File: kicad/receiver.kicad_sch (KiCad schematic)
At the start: 0 parts

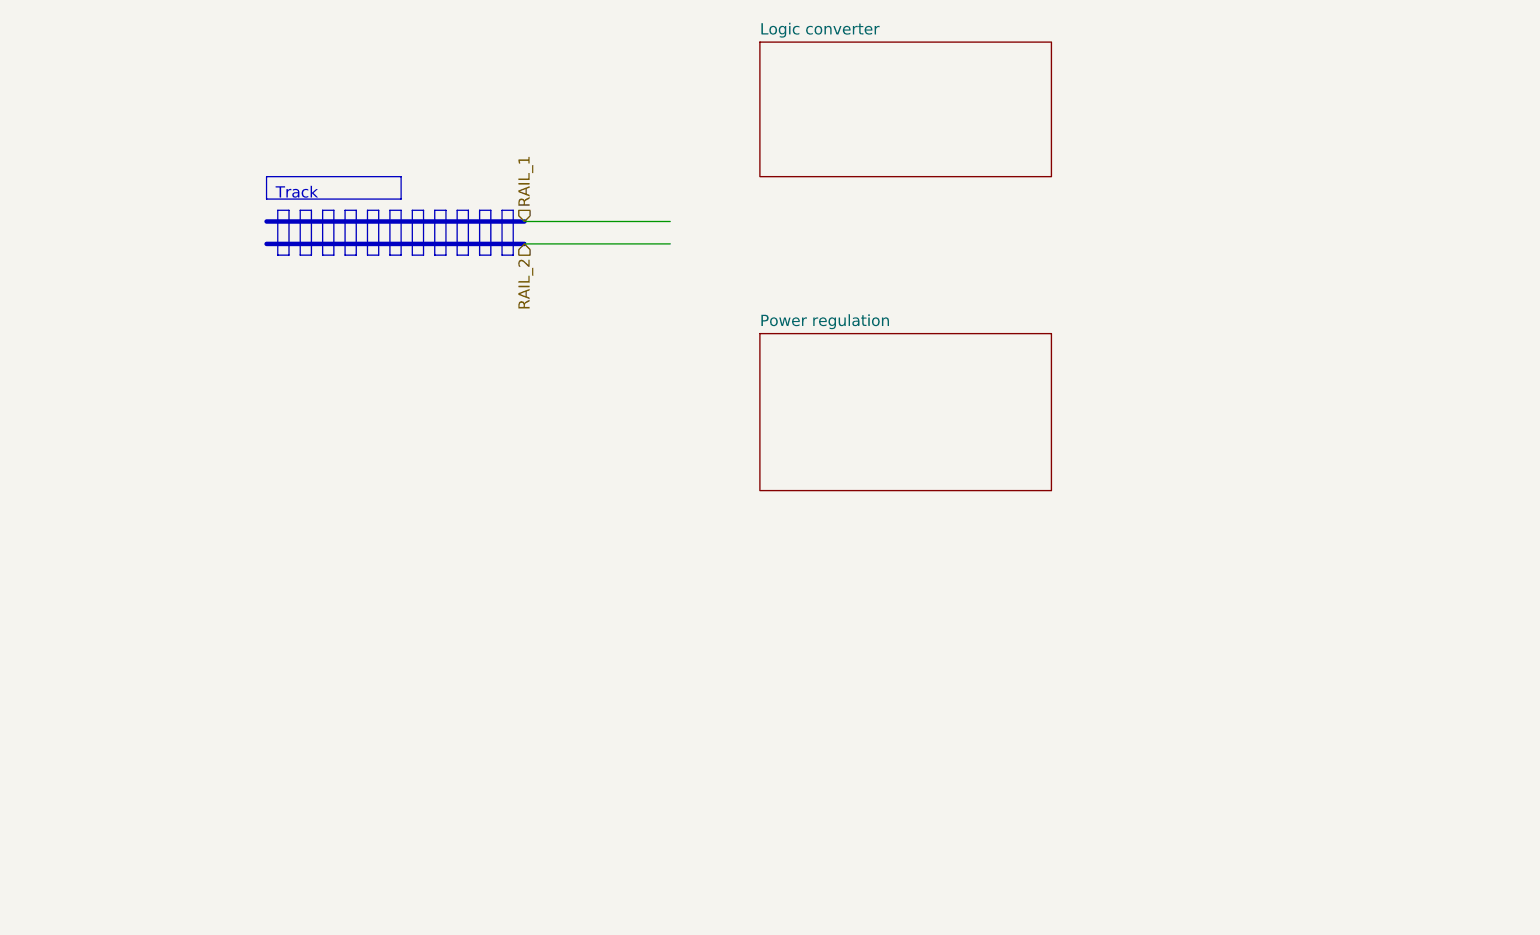
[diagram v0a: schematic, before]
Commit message: split
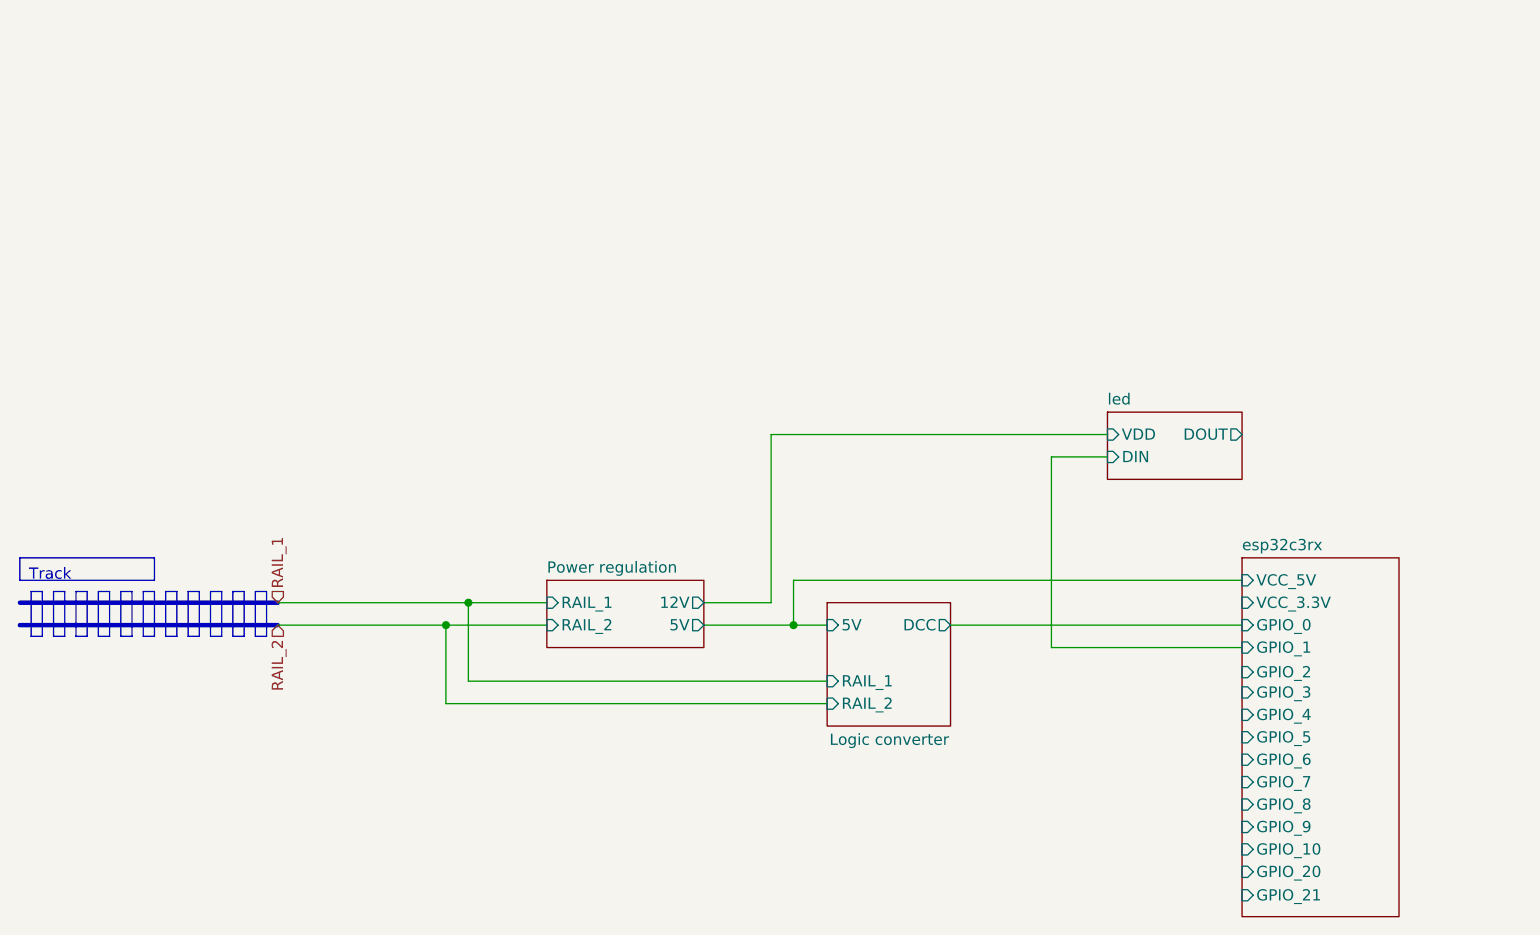
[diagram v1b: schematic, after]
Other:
- added sheet esp32c3rx (esp-c3-rx.kicad_sch)
- added sheet led (led.kicad_sch)
- sheet Logic converter ports: added 5V, DCC, RAIL_1, RAIL_2; removed none
- sheet Power regulation ports: added 12V, 5V, RAIL_1, RAIL_2; removed none

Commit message: kicad changes
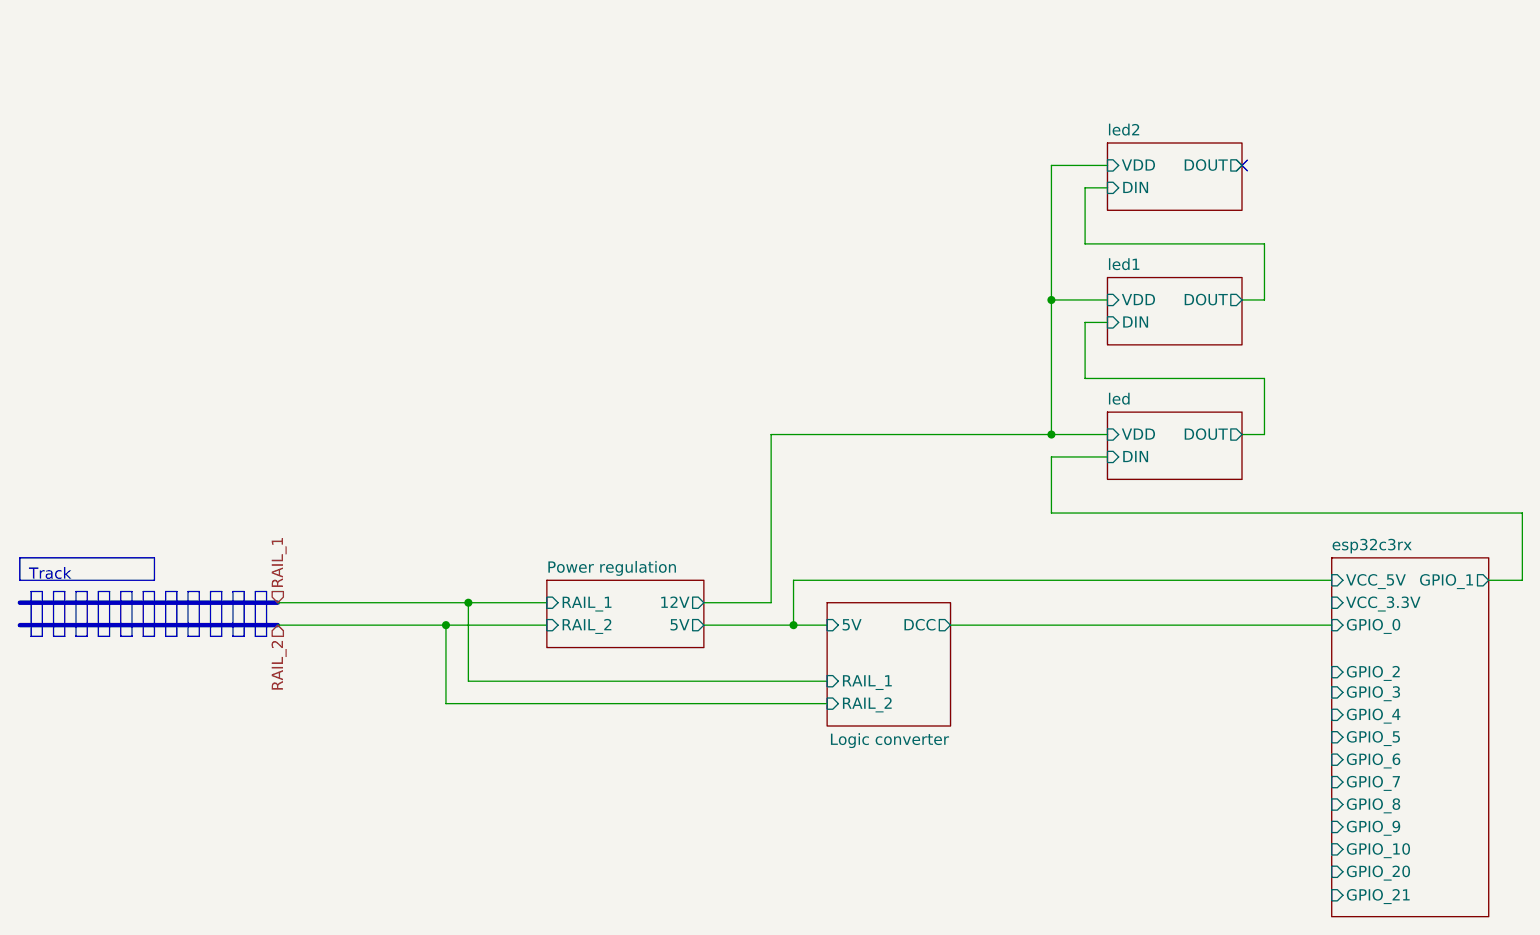
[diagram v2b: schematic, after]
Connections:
- no-connect marks 0 -> 1
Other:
- added sheet led1 (led.kicad_sch)
- added sheet led2 (led.kicad_sch)
